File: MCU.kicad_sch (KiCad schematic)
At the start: 30 parts, among them J10 Conn_01x04, J11 Conn_01x04, J12 Conn_01x03, J6 Conn_01x04, J7 Conn_01x04, J8 Conn_ST_STDC14, J9 Conn_01x03, U15 STM32F303RETx

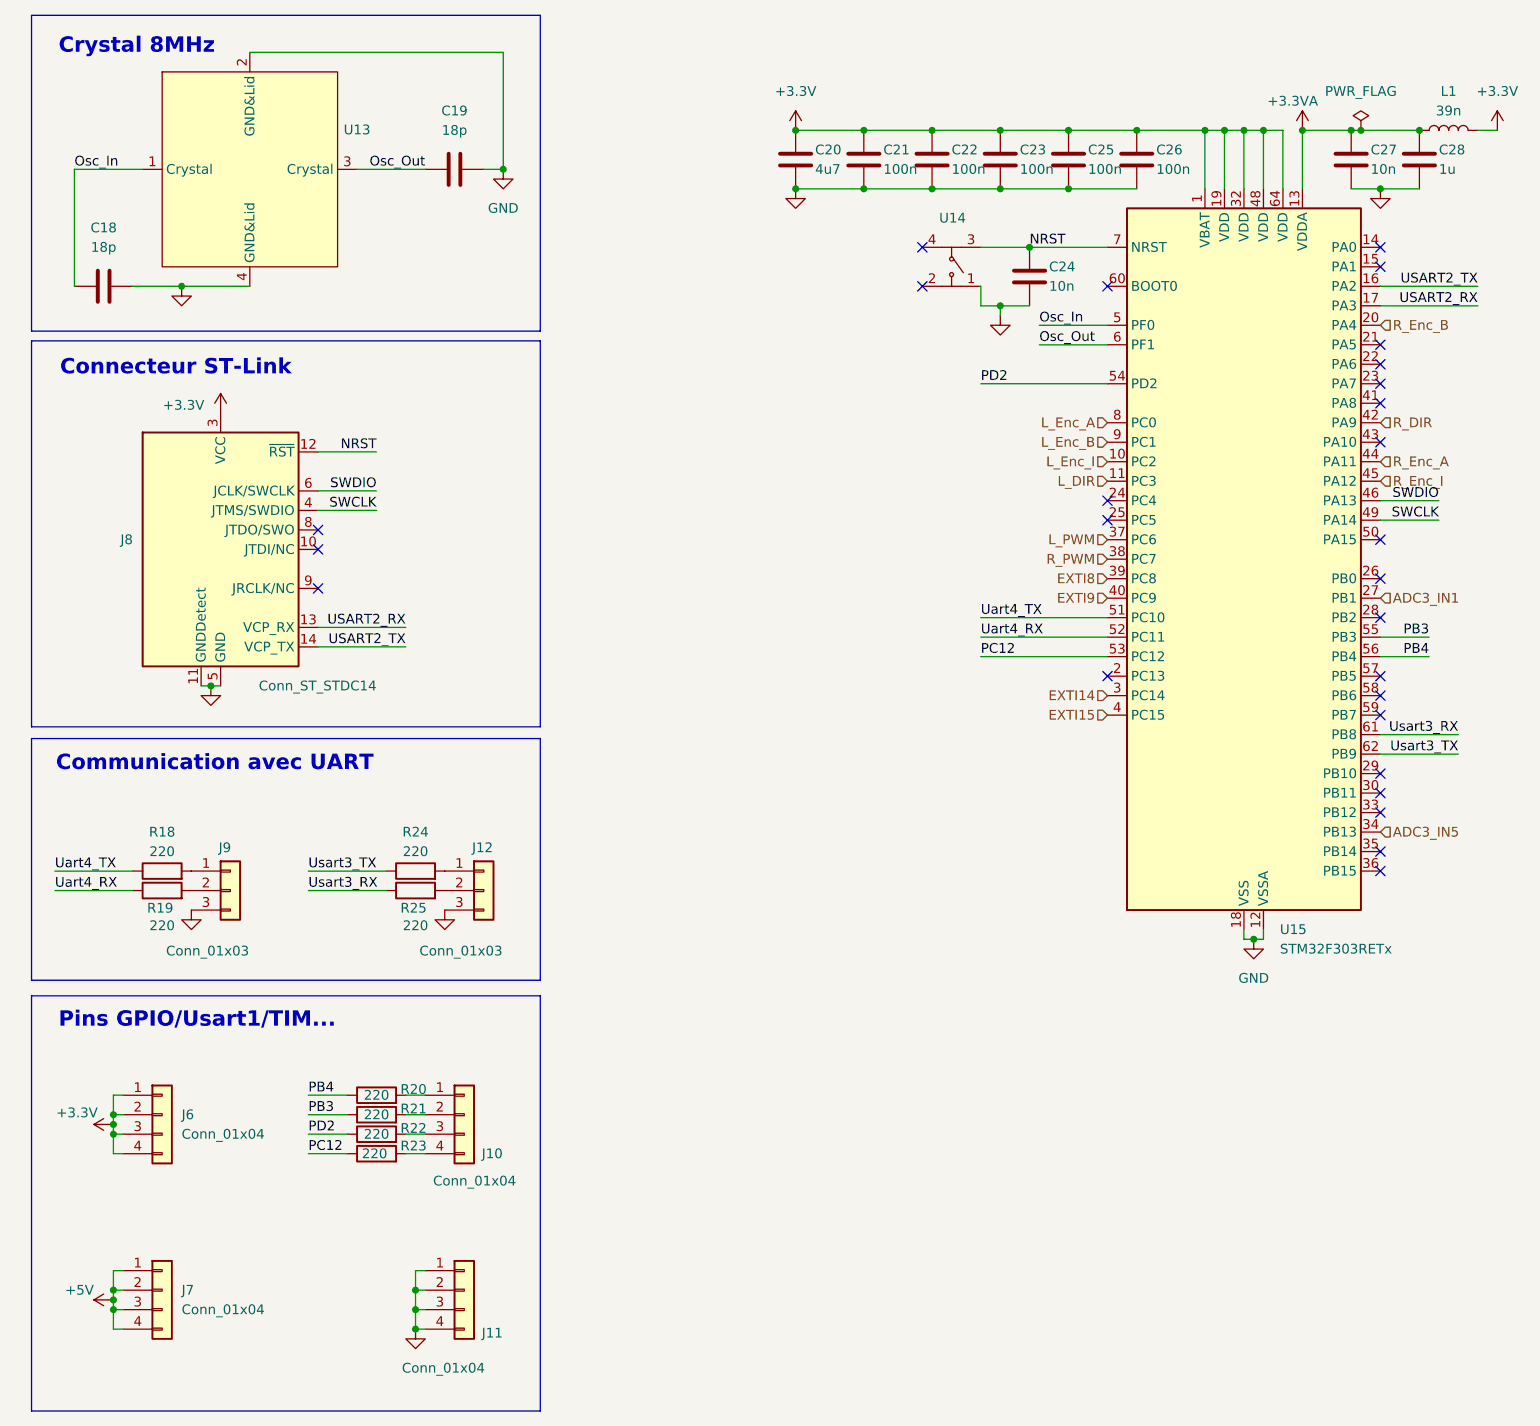
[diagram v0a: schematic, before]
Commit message: maj PCB
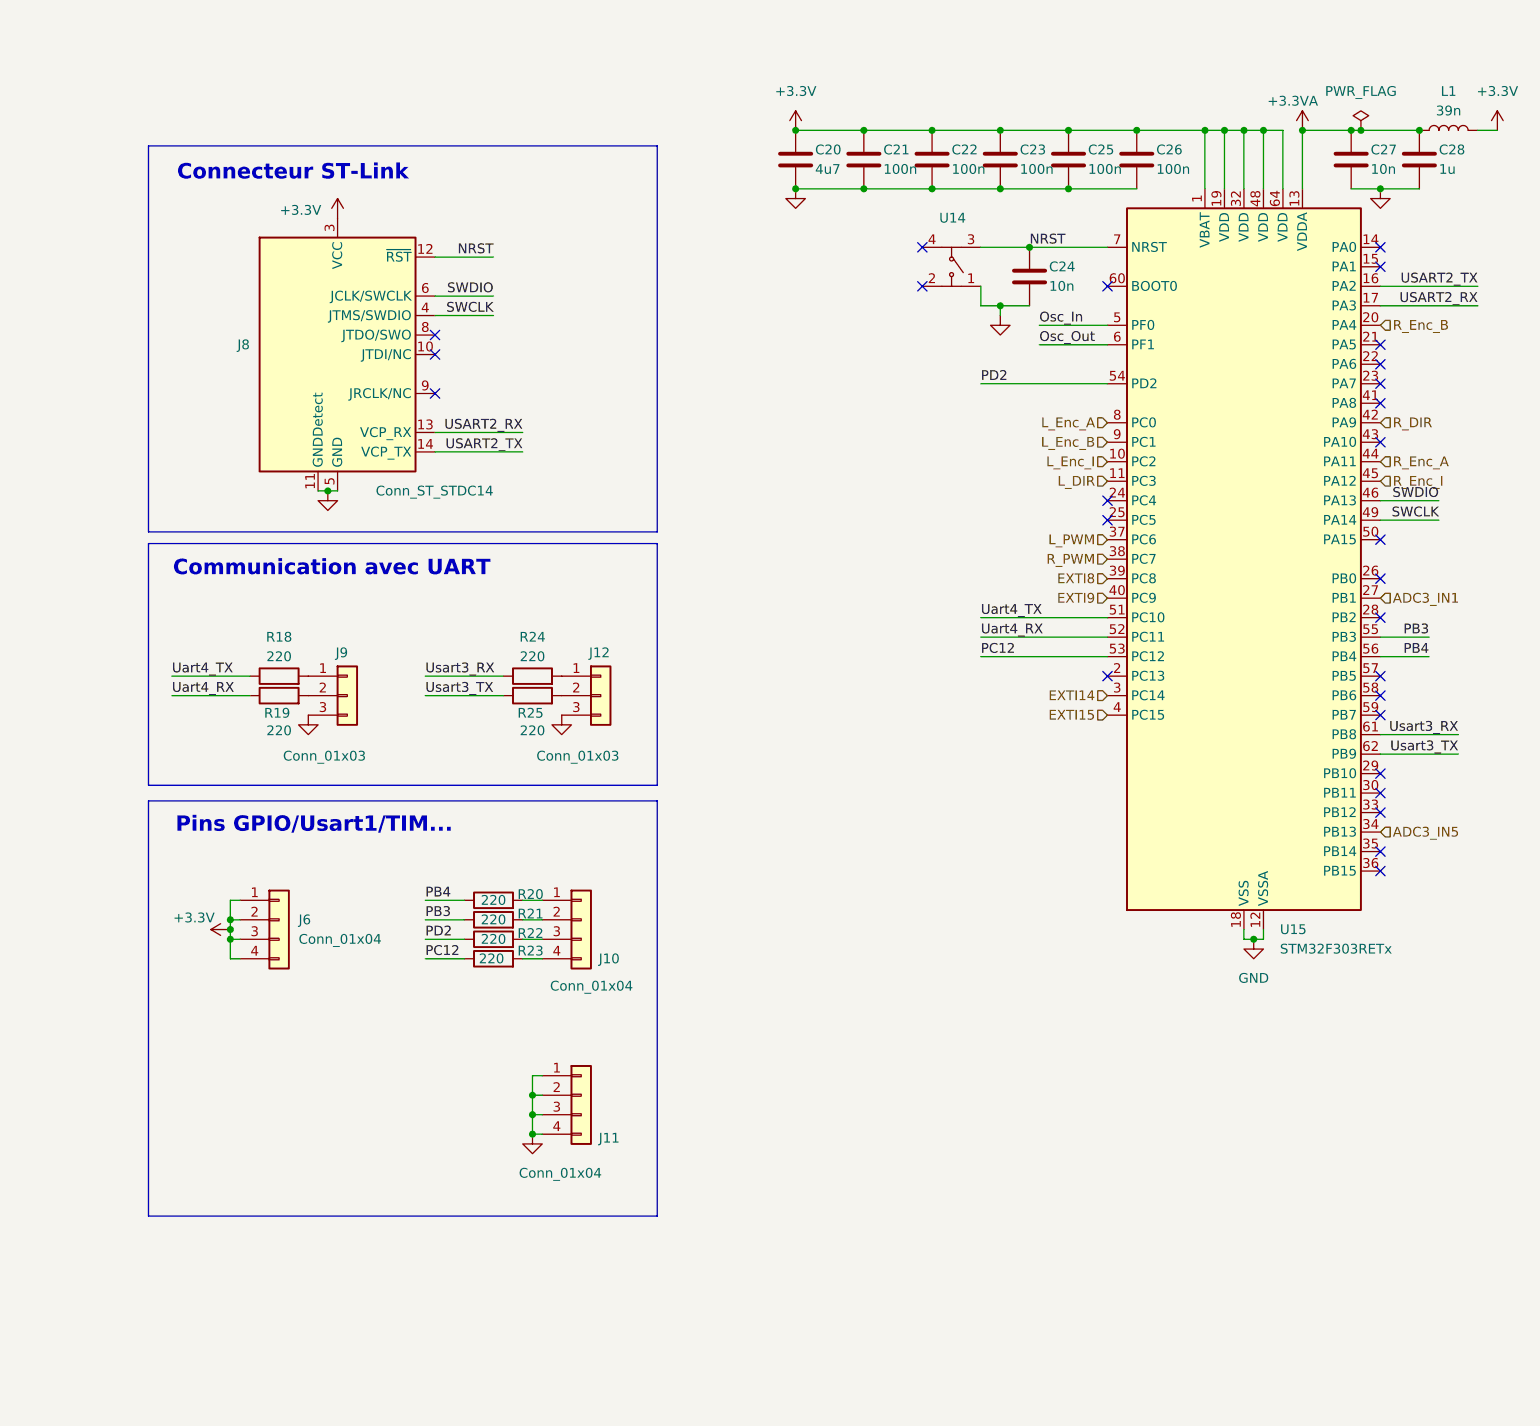
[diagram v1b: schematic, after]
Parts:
- removed C18, C19: 18p, Capacitor_SMD:C_0402_1005Metric, symbol Device:C
- removed J7: Conn_01x04, Connector_PinHeader_2.54mm:PinHeader_1x04_P2.54mm_Vertical, symbol Connector_Generic:Conn_01x04
- removed U13: ~, Oscillator:CFPX-104-8MHz_oscillator, symbol CFPX-104-oscillator:CFPX-104-8MHz-wurth
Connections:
- net Usart3_RX: now also R24.1; no longer R25.1
- net Usart3_TX: now also R25.1; no longer R24.1
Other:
- note removed: "Crystal 8MHz"
- moved on the sheet: J10, J11, J12, J6, J8, J9, R18, R19, R20, R21, R22, R23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
